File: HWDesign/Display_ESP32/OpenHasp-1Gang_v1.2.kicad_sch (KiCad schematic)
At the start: 42 parts, among them J2 Conn_01x04, J5 USB_C_Receptacle_USB2.0, Q1 S8050, Q2 S8050, Q3 S8050, U1 CP2102N-A01-GQFN28, U3 AP2112K-3.3, U4 ESP32-WROOM-32D

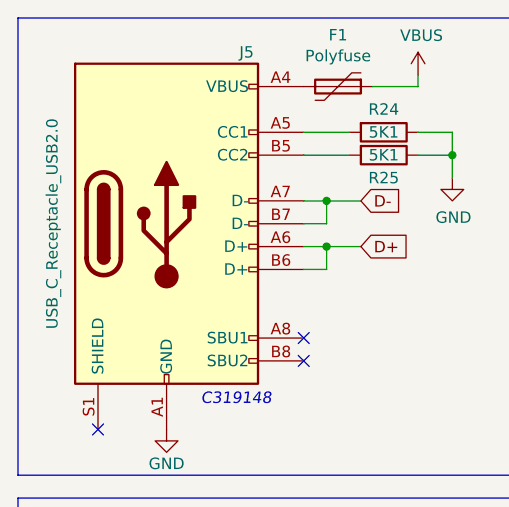
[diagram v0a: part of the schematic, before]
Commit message: Adding gerber/libraryfiles
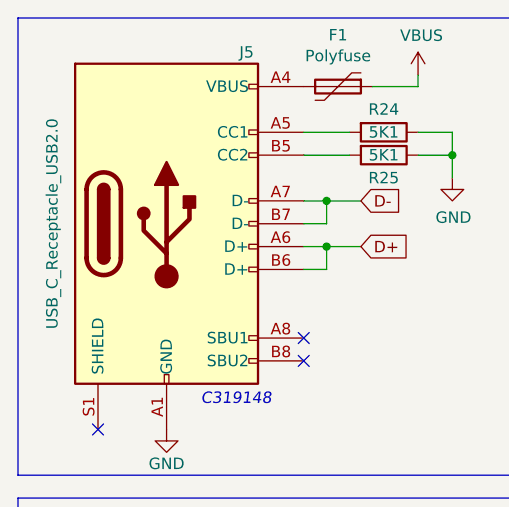
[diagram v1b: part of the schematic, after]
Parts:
- FPC1: footprint ESP32_TouchDown_lib:Hirose_FH12-40S-0.5SH_1x40-1MP_P0.50mm_Horizontal_flipped -> Openhasp:Hirose_FH12-40S-0.5SH_1x40-1MP_P0.50mm_Horizontal_flipped_copy
